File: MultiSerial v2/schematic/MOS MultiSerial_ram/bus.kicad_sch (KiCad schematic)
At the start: 8 parts, among them J12 Conn_01x01, U1 SN74LVCC4245ANSR

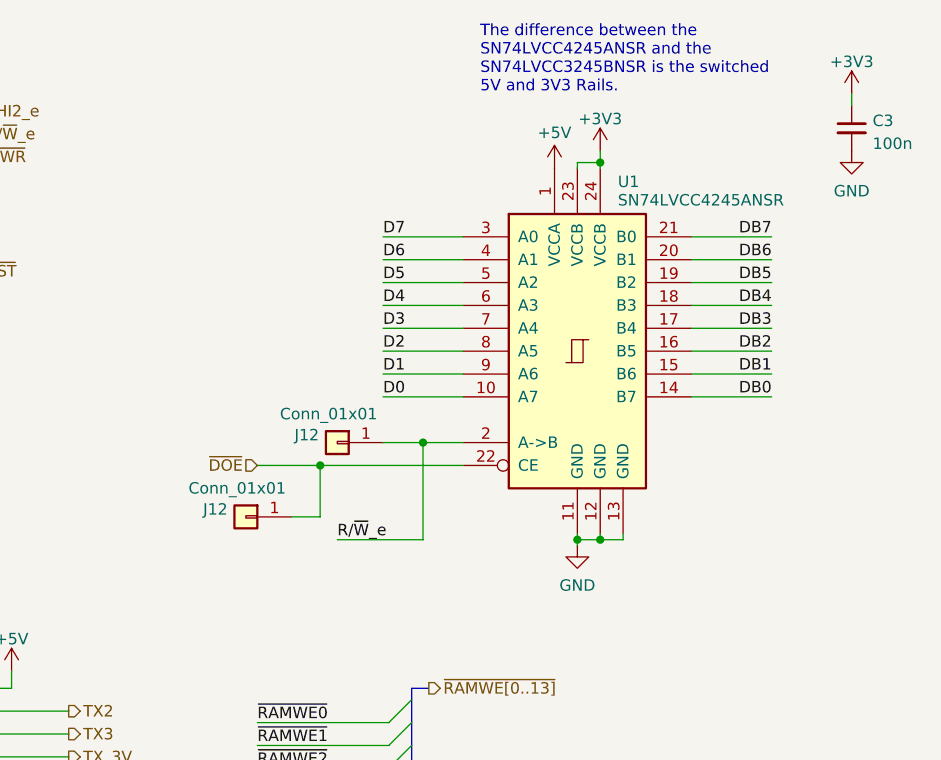
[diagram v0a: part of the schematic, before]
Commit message: python work
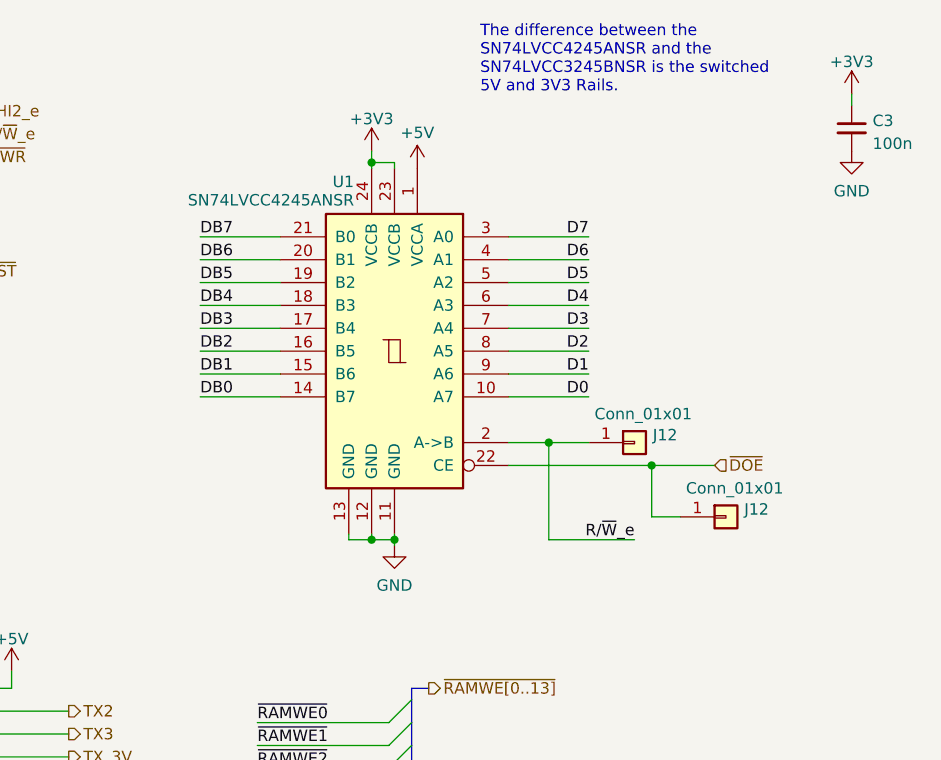
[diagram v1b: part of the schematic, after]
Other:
- moved on the sheet: J12, U1
